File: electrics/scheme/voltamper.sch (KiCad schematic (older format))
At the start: 157 parts, among them K1 swd, K2 servo-1, K3 servo-2, P1 boot, P10 m3-hole, P11 m3-hole, P12 CONN_13X2, P2 boot, P3 -, P4 +, P5 work, P6 aux, P7 ref, P8 m3-hole, P9 m3-hole, Q1 bc857, Q2 bc847, Q3 bc857, Q4 bc847, Q5 irlml2244, Q6 bc847, Q7 bc847, Q8 bc847, SW1 btn-1, SW2 btn-2, U1 CRYSTAL-4PIN, U10 LM258A, U11 INA126, U12 SPARTAN-SIP-9007, U13 OPA551, U14 AD825, U15 AD825, U2 CP2102, U3 MICRO-USB-B, U4 MCP1703T-3302E/CB, U5 MCP1703T-3302E/CB, U6 NCP3063, U7 SPARTAN-SIP-9007, U8 NCP3063

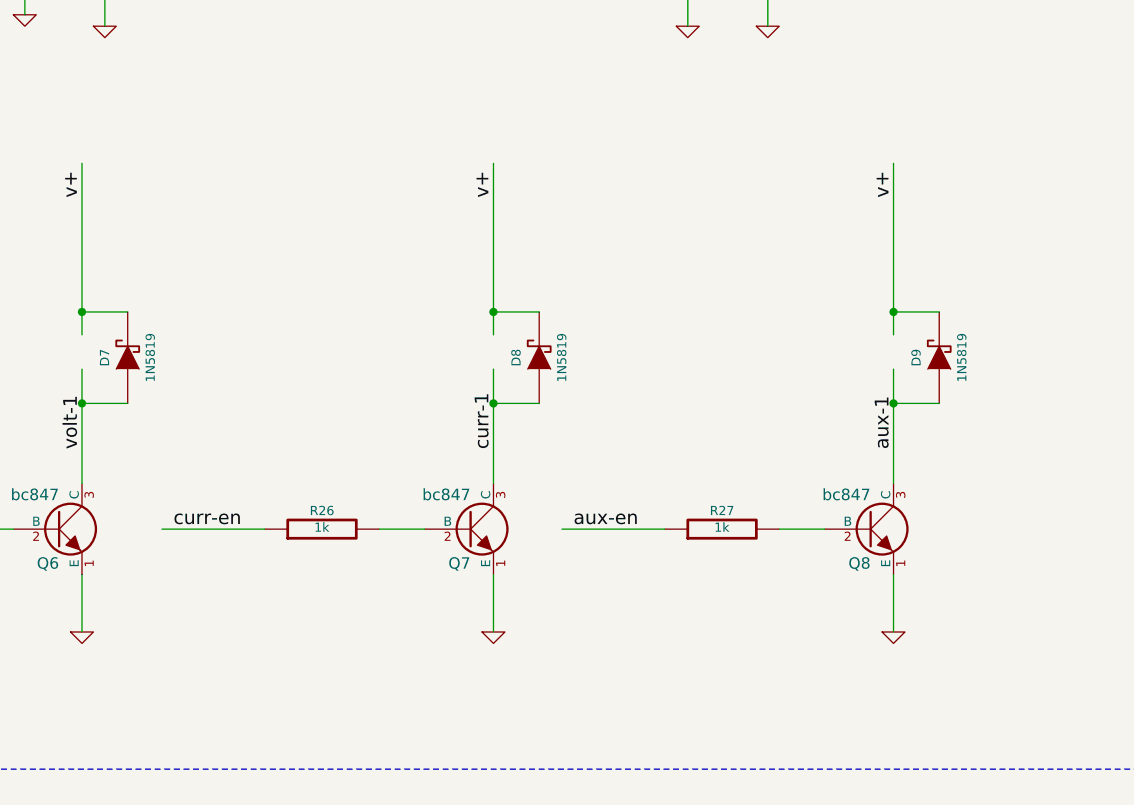
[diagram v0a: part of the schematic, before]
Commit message: a
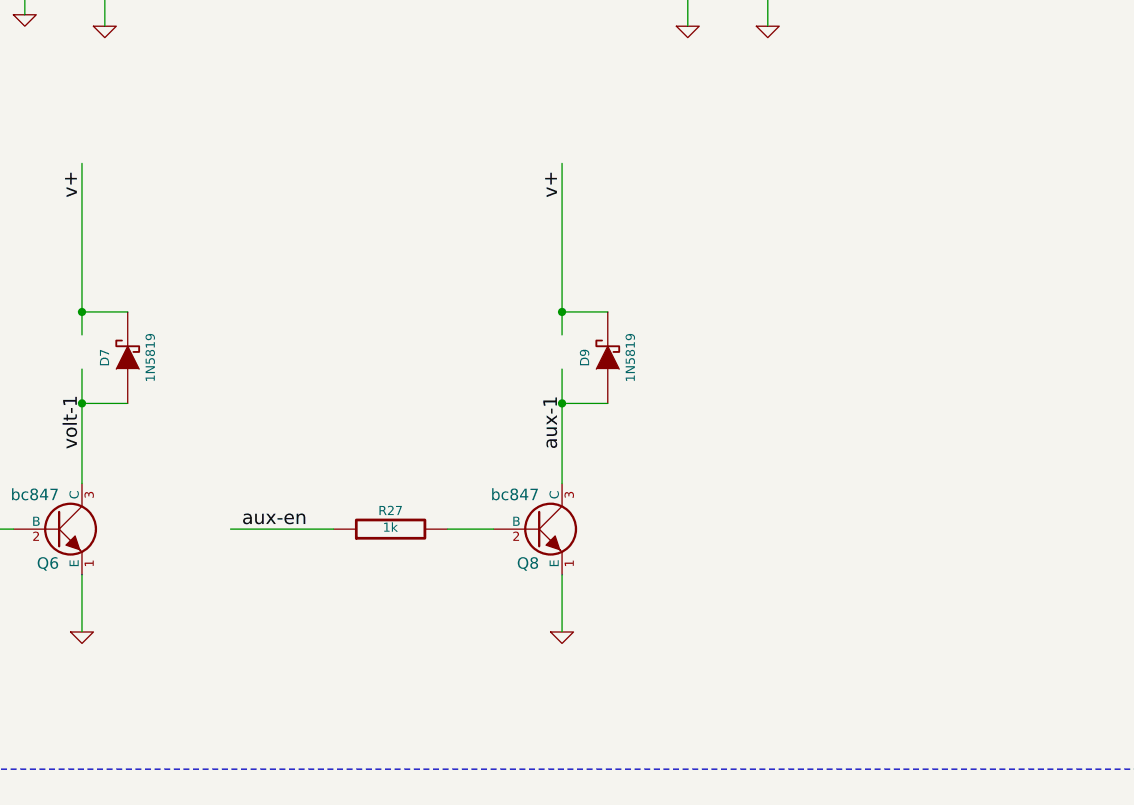
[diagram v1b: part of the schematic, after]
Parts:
- removed D8: 1N5819, ~, symbol DIODESCH
- removed Q7: bc847, ~, symbol NPN
- removed R26: 1k, ~, symbol R
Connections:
- net labels removed: curr-1
- wire segments 520 -> 513
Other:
- moved on the sheet: D9, Q8, R27
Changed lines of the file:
@@
 Sheet 1 1
 Title ""
-Date "1 jan 2015"
+Date "2 jan 2015"
 Rev ""
 Comp ""
@@
 volt-en
 $Comp
-L NPN Q7
-U 1 1 548613CB
-P 11800 18900
-F 0 "Q7" H 11800 18750 50  0000 R CNN
-F 1 "bc847" H 11800 19050 50  0000 R CNN
-F 2 "~" H 11800 18900 60  0000 C CNN
-F 3 "~" H 11800 18900 60  0000 C CNN
-	1    11800 18900
-	1    0    0    -1
-$EndComp
-$Comp
-L R R26
-U 1 1 548613D1
-P 11150 18900
-F 0 "R26" V 11230 18900 40  0000 C CNN
-F 1 "1k" V 11157 18901 40  0000 C CNN
-F 2 "~" V 11080 18900 30  0000 C CNN
-F 3 "~" H 11150 18900 30  0000 C CNN
-	1    11150 18900
-	0    -1   -1   0
-$EndComp
-Wire Wire Line
-	11600 18900 11400 18900
-Wire Wire Line
-	11900 18700 11900 18200
-Wire Wire Line
-	11900 19100 11900 19350
-$Comp
-L GND #PWR055
-U 1 1 548613DA
-P 11900 19350
-F 0 "#PWR055" H 11900 19350 30  0001 C CNN
-F 1 "GND" H 11900 19280 30  0001 C CNN
-F 2 "" H 11900 19350 60  0000 C CNN
-F 3 "" H 11900 19350 60  0000 C CNN
-	1    11900 19350
-	1    0    0    -1
-$EndComp
-Wire Wire Line
-	10900 18900 10450 18900
-Text Label 11900 18550 1    60   ~ 0
-curr-1
-Wire Wire Line
-	11900 17300 11900 18050
-Text Label 11900 17450 1    60   ~ 0
-v+
-Text Label 10500 18900 0    60   ~ 0
-curr-en
-$Comp
 L NPN Q8
 U 1 1 548615B1
-P 13550 18900
-F 0 "Q8" H 13550 18750 50  0000 R CNN
-F 1 "bc847" H 13550 19050 50  0000 R CNN
-F 2 "~" H 13550 18900 60  0000 C CNN
-F 3 "~" H 13550 18900 60  0000 C CNN
-	1    13550 18900
+P 12100 18900
+F 0 "Q8" H 12100 18750 50  0000 R CNN
+F 1 "bc847" H 12100 19050 50  0000 R CNN
+F 2 "~" H 12100 18900 60  0000 C CNN
+F 3 "~" H 12100 18900 60  0000 C CNN
+	1    12100 18900
 	1    0    0    -1
 $EndComp
@@
 L R R27
 U 1 1 548615B7
-P 12900 18900
-F 0 "R27" V 12980 18900 40  0000 C CNN
-F 1 "1k" V 12907 18901 40  0000 C CNN
-F 2 "~" V 12830 18900 30  0000 C CNN
-F 3 "~" H 12900 18900 30  0000 C CNN
-	1    12900 18900
+P 11450 18900
+F 0 "R27" V 11530 18900 40  0000 C CNN
+F 1 "1k" V 11457 18901 40  0000 C CNN
+F 2 "~" V 11380 18900 30  0000 C CNN
+F 3 "~" H 11450 18900 30  0000 C CNN
+	1    11450 18900
 	0    -1   -1   0
 $EndComp
 Wire Wire Line
-	13350 18900 13150 18900
-Wire Wire Line
-	13650 18700 13650 18200
-Wire Wire Line
-	13650 19100 13650 19350
+	11900 18900 11700 18900
+Wire Wire Line
+	12200 18700 12200 18200
+Wire Wire Line
+	12200 19100 12200 19350
 $Comp
 L GND #PWR056
 U 1 1 548615C0
-P 13650 19350
-F 0 "#PWR056" H 13650 19350 30  0001 C CNN
-F 1 "GND" H 13650 19280 30  0001 C CNN
-F 2 "" H 13650 19350 60  0000 C CNN
-F 3 "" H 13650 19350 60  0000 C CNN
-	1    13650 19350
-	1    0    0    -1
-$EndComp
-Wire Wire Line
-	12650 18900 12200 18900
-Text Label 13650 18550 1    60   ~ 0
+P 12200 19350
+F 0 "#PWR056" H 12200 19350 30  0001 C CNN
+F 1 "GND" H 12200 19280 30  0001 C CNN
+F 2 "" H 12200 19350 60  0000 C CNN
+F 3 "" H 12200 19350 60  0000 C CNN
+	1    12200 19350
+	1    0    0    -1
+$EndComp
+Wire Wire Line
+	11200 18900 10750 18900
+Text Label 12200 18550 1    60   ~ 0
 aux-1
 Wire Wire Line
-	13650 17300 13650 18050
-Text Label 13650 17450 1    60   ~ 0
+	12200 17300 12200 18050
+Text Label 12200 17450 1    60   ~ 0
 v+
-Text Label 12250 18900 0    60   ~ 0
+Text Label 10800 18900 0    60   ~ 0
 aux-en
 $Comp
@@
 Connection ~ 10100 18350
 $Comp
-L DIODESCH D8
-U 1 1 5485E6E8
-P 12100 18150
-F 0 "D8" H 12100 18250 40  0000 C CNN
-F 1 "1N5819" H 12100 18050 40  0000 C CNN
-F 2 "~" H 12100 18150 60  0000 C CNN
-F 3 "~" H 12100 18150 60  0000 C CNN
-	1    12100 18150
-	0    -1   -1   0
-$EndComp
-Wire Wire Line
-	12100 17950 11900 17950
-Connection ~ 11900 17950
-Wire Wire Line
-	12100 18350 11900 18350
-Connection ~ 11900 18350
-$Comp
 L DIODESCH D9
 U 1 1 5485EACA
-P 13850 18150
-F 0 "D9" H 13850 18250 40  0000 C CNN
-F 1 "1N5819" H 13850 18050 40  0000 C CNN
-F 2 "~" H 13850 18150 60  0000 C CNN
-F 3 "~" H 13850 18150 60  0000 C CNN
-	1    13850 18150
+P 12400 18150
+F 0 "D9" H 12400 18250 40  0000 C CNN
+F 1 "1N5819" H 12400 18050 40  0000 C CNN
+F 2 "~" H 12400 18150 60  0000 C CNN
+F 3 "~" H 12400 18150 60  0000 C CNN
+	1    12400 18150
 	0    -1   -1   0
 $EndComp
 Wire Wire Line
-	13850 17950 13650 17950
-Connection ~ 13650 17950
-Wire Wire Line
-	13850 18350 13650 18350
-Connection ~ 13650 18350
+	12400 17950 12200 17950
+Connection ~ 12200 17950
+Wire Wire Line
+	12400 18350 12200 18350
+Connection ~ 12200 18350
 $Comp
 L LED D10
